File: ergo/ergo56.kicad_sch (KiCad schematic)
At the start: 129 parts, among them J1 BAT, J2 AudioJack3_Ground, J3 AudioJack3_Ground, J5 Conn_ARM_SWD, U1 PCA9555PW, U2 Seeeduino Xiao nRF52840

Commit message: all today
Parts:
- H1, H2, H3, H4, H5, H6, H7, H8: footprint (none) -> MountingHole:MountingHole_3.5mm
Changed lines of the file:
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@@
       (effects (font (size 1.27 1.27)) (justify left))
     )
-    (property "Footprint" "" (at 267.97 141.605 0)
+    (property "Footprint" "MountingHole:MountingHole_3.5mm" (at 267.97 141.605 0)
       (effects (font (size 1.27 1.27)) hide)
     )
@@
       (effects (font (size 1.27 1.27)) (justify left) hide)
     )
-    (property "Footprint" "" (at 267.97 159.385 0)
+    (property "Footprint" "MountingHole:MountingHole_3.5mm" (at 267.97 159.385 0)
       (effects (font (size 1.27 1.27)) hide)
     )
@@
       (effects (font (size 1.27 1.27)) (justify left) hide)
     )
-    (property "Footprint" "" (at 275.59 147.32 0)
+    (property "Footprint" "MountingHole:MountingHole_3.5mm" (at 275.59 147.32 0)
       (effects (font (size 1.27 1.27)) hide)
     )
@@
       (effects (font (size 1.27 1.27)) (justify left) hide)
     )
-    (property "Footprint" "" (at 275.59 153.67 0)
+    (property "Footprint" "MountingHole:MountingHole_3.5mm" (at 275.59 153.67 0)
       (effects (font (size 1.27 1.27)) hide)
     )
@@
       (effects (font (size 1.27 1.27)) (justify left) hide)
     )
-    (property "Footprint" "" (at 267.97 153.67 0)
+    (property "Footprint" "MountingHole:MountingHole_3.5mm" (at 267.97 153.67 0)
       (effects (font (size 1.27 1.27)) hide)
     )
@@
       (effects (font (size 1.27 1.27)) (justify left) hide)
     )
-    (property "Footprint" "" (at 275.59 141.605 0)
+    (property "Footprint" "MountingHole:MountingHole_3.5mm" (at 275.59 141.605 0)
       (effects (font (size 1.27 1.27)) hide)
     )
@@
       (effects (font (size 1.27 1.27)) (justify left) hide)
     )
-    (property "Footprint" "" (at 275.59 159.385 0)
+    (property "Footprint" "MountingHole:MountingHole_3.5mm" (at 275.59 159.385 0)
       (effects (font (size 1.27 1.27)) hide)
     )
@@
       (effects (font (size 1.27 1.27)) (justify left) hide)
     )
-    (property "Footprint" "" (at 267.97 147.32 0)
-      (effects (font (size 1.27 1.27)) hide)
-    )
+    (property "Footprint" "MountingHole:MountingHole_3.5mm" (at 267.97 147.32 0)
+      (effects (font (size 1.27 1.27)) hide)
+    )

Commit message: stage
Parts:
- U2: footprint PCM_marbastlib-xp-promicroish:Xiao_nRF52840_ACH -> PCM_marbastlib-xp-promicroish:Xiao_nRF52840_AC_Reflow
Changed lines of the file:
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@@
       (effects (font (size 1.27 1.27)) (justify left))
     )
-    (property "Footprint" "PCM_marbastlib-xp-promicroish:Xiao_nRF52840_ACH" (at 49.53 179.07 0)
+    (property "Footprint" "PCM_marbastlib-xp-promicroish:Xiao_nRF52840_AC_Reflow" (at 49.53 179.07 0)
       (effects (font (size 1.27 1.27)) hide)
     )

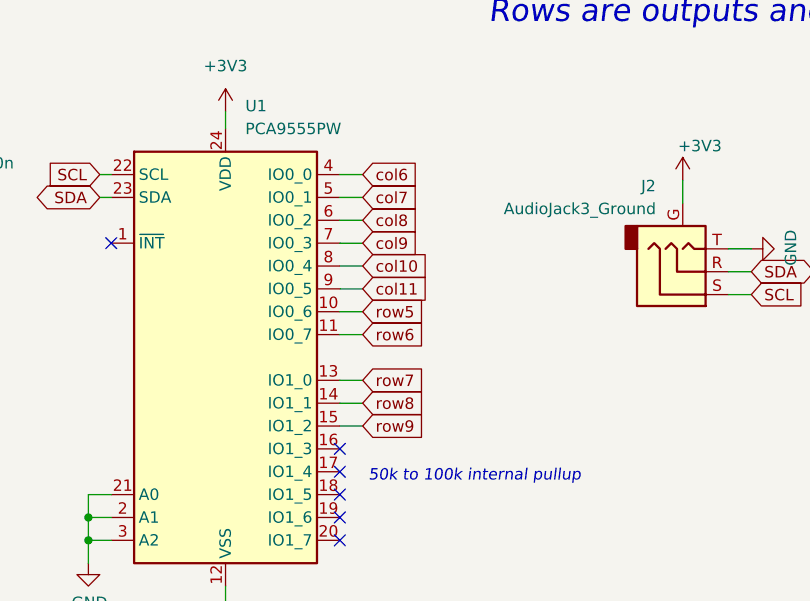
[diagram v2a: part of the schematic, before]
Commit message: finish pcb
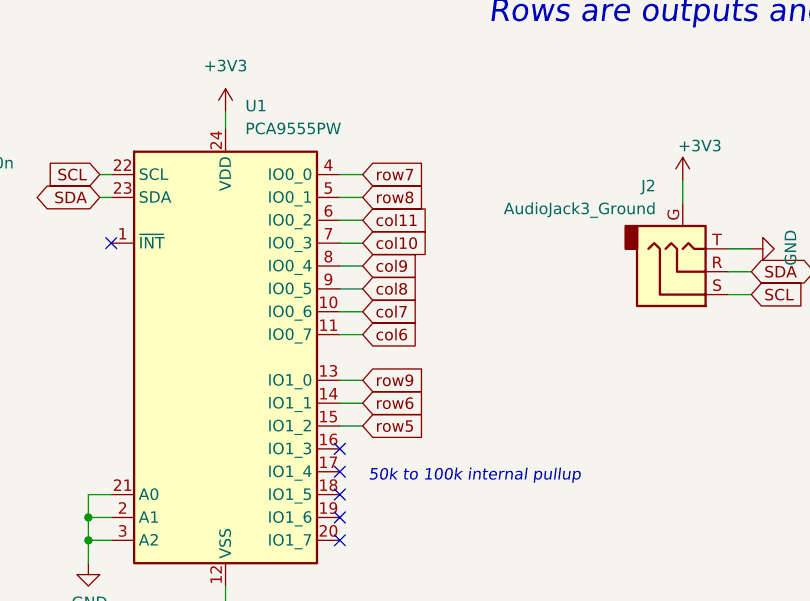
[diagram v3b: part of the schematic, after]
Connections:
- net col10: now also U1.7 (IO0_3); no longer U1.8 (IO0_4)
- net col11: now also U1.6 (IO0_2); no longer U1.9 (IO0_5)
- net col6: now also U1.11 (IO0_7); no longer U1.4 (IO0_0)
- net col7: now also U1.10 (IO0_6); no longer U1.5 (IO0_1)
- net col8: now also U1.9 (IO0_5); no longer U1.6 (IO0_2)
- net col9: now also U1.8 (IO0_4); no longer U1.7 (IO0_3)
- net row5: now also U1.15 (IO1_2); no longer U1.10 (IO0_6)
- net row6: now also U1.14 (IO1_1); no longer U1.11 (IO0_7)
- net row7: now also U1.4 (IO0_0); no longer U1.13 (IO1_0)
- net row8: now also U1.5 (IO0_1); no longer U1.14 (IO1_1)
- net row9: now also U1.13 (IO1_0); no longer U1.15 (IO1_2)
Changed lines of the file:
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@@
     (effects (font (size 2.5 2.5) italic) (justify left bottom))
   )
-  (global_label "col6" (shape input) (at 139.7 133.985 0) (fields_autoplaced)
-    (effects (font (size 1.27 1.27)) (justify left))
-    (property "Intersheetrefs" "${INTERSHEET_REFS}" (at 146.1433 133.985 0)
+  (global_label "col6" (shape input) (at 139.7 151.765 0) (fields_autoplaced)
+    (effects (font (size 1.27 1.27)) (justify left))
+    (property "Intersheetrefs" "${INTERSHEET_REFS}" (at 146.1433 151.765 0)
       (effects (font (size 1.27 1.27)) (justify left) hide)
     )
@@
     )
   )
-  (global_label "col8" (shape input) (at 139.7 139.065 0) (fields_autoplaced)
-    (effects (font (size 1.27 1.27)) (justify left))
-    (property "Intersheetrefs" "${INTERSHEET_REFS}" (at 146.1433 139.065 0)
+  (global_label "col8" (shape input) (at 139.7 146.685 0) (fields_autoplaced)
+    (effects (font (size 1.27 1.27)) (justify left))
+    (property "Intersheetrefs" "${INTERSHEET_REFS}" (at 146.1433 146.685 0)
       (effects (font (size 1.27 1.27)) (justify left) hide)
     )
@@
     )
   )
-  (global_label "col11" (shape input) (at 139.7 146.685 0) (fields_autoplaced)
-    (effects (font (size 1.27 1.27)) (justify left))
-    (property "Intersheetrefs" "${INTERSHEET_REFS}" (at 147.3528 146.685 0)
-      (effects (font (size 1.27 1.27)) (justify left) hide)
-    )
-  )
-  (global_label "row5" (shape input) (at 139.7 149.225 0) (fields_autoplaced)
-    (effects (font (size 1.27 1.27)) (justify left))
-    (property "Intersheetrefs" "${INTERSHEET_REFS}" (at 146.5062 149.225 0)
+  (global_label "col11" (shape input) (at 139.7 139.065 0) (fields_autoplaced)
+    (effects (font (size 1.27 1.27)) (justify left))
+    (property "Intersheetrefs" "${INTERSHEET_REFS}" (at 147.3528 139.065 0)
+      (effects (font (size 1.27 1.27)) (justify left) hide)
+    )
+  )
+  (global_label "row5" (shape input) (at 139.7 161.925 0) (fields_autoplaced)
+    (effects (font (size 1.27 1.27)) (justify left))
+    (property "Intersheetrefs" "${INTERSHEET_REFS}" (at 146.5062 161.925 0)
       (effects (font (size 1.27 1.27)) (justify left) hide)
     )
@@
     )
   )
-  (global_label "row7" (shape input) (at 139.7 156.845 0) (fields_autoplaced)
-    (effects (font (size 1.27 1.27)) (justify left))
-    (property "Intersheetrefs" "${INTERSHEET_REFS}" (at 146.5062 156.845 0)
+  (global_label "row7" (shape input) (at 139.7 133.985 0) (fields_autoplaced)
+    (effects (font (size 1.27 1.27)) (justify left))
+    (property "Intersheetrefs" "${INTERSHEET_REFS}" (at 146.5062 133.985 0)
       (effects (font (size 1.27 1.27)) (justify left) hide)
     )
@@
     )
   )
-  (global_label "row9" (shape input) (at 139.7 161.925 0) (fields_autoplaced)
-    (effects (font (size 1.27 1.27)) (justify left))
-    (property "Intersheetrefs" "${INTERSHEET_REFS}" (at 146.5062 161.925 0)
+  (global_label "row9" (shape input) (at 139.7 156.845 0) (fields_autoplaced)
+    (effects (font (size 1.27 1.27)) (justify left))
+    (property "Intersheetrefs" "${INTERSHEET_REFS}" (at 146.5062 156.845 0)
       (effects (font (size 1.27 1.27)) (justify left) hide)
     )
@@
     )
   )
-  (global_label "col9" (shape input) (at 139.7 141.605 0) (fields_autoplaced)
-    (effects (font (size 1.27 1.27)) (justify left))
-    (property "Intersheetrefs" "${INTERSHEET_REFS}" (at 146.1433 141.605 0)
+  (global_label "col9" (shape input) (at 139.7 144.145 0) (fields_autoplaced)
+    (effects (font (size 1.27 1.27)) (justify left))
+    (property "Intersheetrefs" "${INTERSHEET_REFS}" (at 146.1433 144.145 0)
       (effects (font (size 1.27 1.27)) (justify left) hide)
     )
@@
     )
   )
-  (global_label "col10" (shape input) (at 139.7 144.145 0) (fields_autoplaced)
-    (effects (font (size 1.27 1.27)) (justify left))
-    (property "Intersheetrefs" "${INTERSHEET_REFS}" (at 147.3528 144.145 0)
+  (global_label "col10" (shape input) (at 139.7 141.605 0) (fields_autoplaced)
+    (effects (font (size 1.27 1.27)) (justify left))
+    (property "Intersheetrefs" "${INTERSHEET_REFS}" (at 147.3528 141.605 0)
       (effects (font (size 1.27 1.27)) (justify left) hide)
     )
@@
     )
   )
-  (global_label "row6" (shape input) (at 139.7 151.765 0) (fields_autoplaced)
-    (effects (font (size 1.27 1.27)) (justify left))
-    (property "Intersheetrefs" "${INTERSHEET_REFS}" (at 146.5062 151.765 0)
-      (effects (font (size 1.27 1.27)) (justify left) hide)
-    )
-  )
-  (global_label "col7" (shape input) (at 139.7 136.525 0) (fields_autoplaced)
-    (effects (font (size 1.27 1.27)) (justify left))
-    (property "Intersheetrefs" "${INTERSHEET_REFS}" (at 146.1433 136.525 0)
+  (global_label "row6" (shape input) (at 139.7 159.385 0) (fields_autoplaced)
+    (effects (font (size 1.27 1.27)) (justify left))
+    (property "Intersheetrefs" "${INTERSHEET_REFS}" (at 146.5062 159.385 0)
+      (effects (font (size 1.27 1.27)) (justify left) hide)
+    )
+  )
+  (global_label "col7" (shape input) (at 139.7 149.225 0) (fields_autoplaced)
+    (effects (font (size 1.27 1.27)) (justify left))
+    (property "Intersheetrefs" "${INTERSHEET_REFS}" (at 146.1433 149.225 0)
       (effects (font (size 1.27 1.27)) (justify left) hide)
     )
@@
     )
   )
-  (global_label "row8" (shape input) (at 139.7 159.385 0) (fields_autoplaced)
-    (effects (font (size 1.27 1.27)) (justify left))
-    (property "Intersheetrefs" "${INTERSHEET_REFS}" (at 146.5062 159.385 0)
-      (effects (font (size 1.27 1.27)) (justify left) hide)
-    )
+  (global_label "row8" (shape input) (at 139.7 136.525 0) (fields_autoplaced)
+    (effects (font (size 1.27 1.27)) (justify left))
+    (property "Intersheetrefs" "${INTERSHEET_REFS}" (at 146.5062 136.525 0)
+      (effects (font (size 1.27 1.27)) (justify left) hide)
+    )
